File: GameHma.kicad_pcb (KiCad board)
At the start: 2 copper layers, 14 parts, among them J2 Motor_Terminal_01x04, J3 Motor_Terminal_01x04, J4 Motor_Terminal_01x04, J5 Motor_Terminal_01x04, U1 ESP32-DEVKIT-V1, U2 A4988_STEPPER_MOTOR_DRIVER_CA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, U3 A4988_STEPPER_MOTOR_DRIVER_CA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, U4 A4988_STEPPER_MOTOR_DRIVER_CA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, U5 A4988_STEPPER_MOTOR_DRIVER_CA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, U6 SRT_MP1584EN

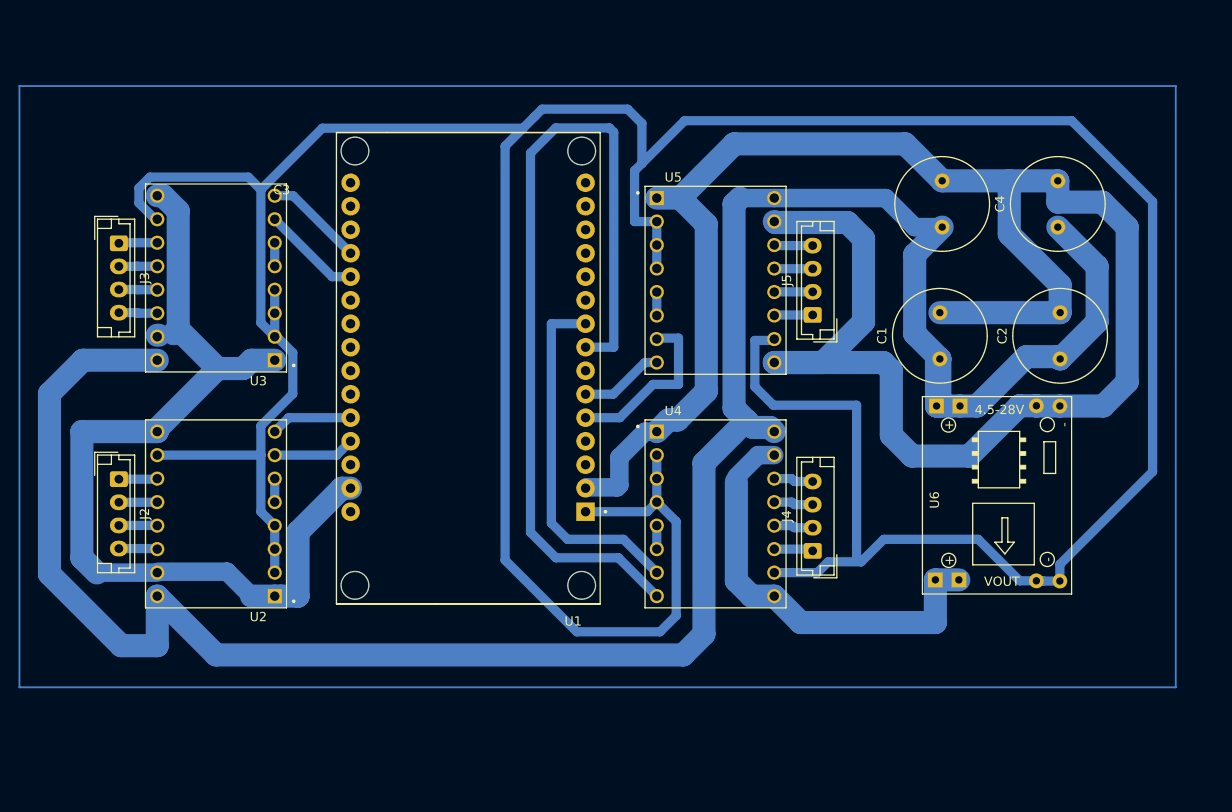
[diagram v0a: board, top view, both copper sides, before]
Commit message: Add log, Finish PCB rout line
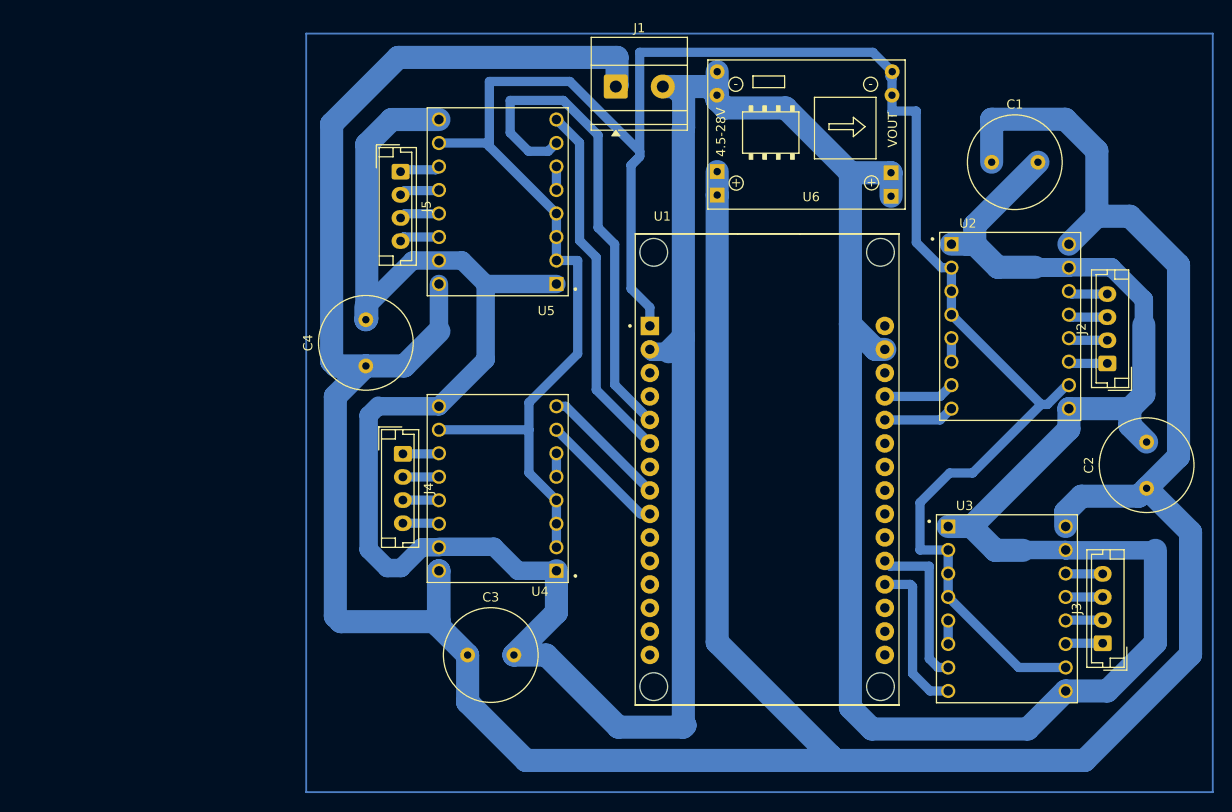
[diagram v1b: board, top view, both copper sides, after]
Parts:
- added J1: Screw_Terminal_01x02, TerminalBlock_Phoenix:TerminalBlock_Phoenix_MKDS-1,5-2-5.08_1x02_P5.08mm_Horizontal, F.Cu at (130.2, 64.8)
- moved J3 114.8 mm to (182.8, 125.0), turned to 90 degrees
- moved J2 107.6 mm to (183.3, 94.7), turned to 90 degrees
- moved U3 92.7 mm to (172.5, 121.3), turned to 0 degrees
- moved U2 88.2 mm to (172.8, 90.7), turned to 0 degrees
- moved C4 76.3 mm to (103.2, 95.0)
- moved C3 69.1 mm to (114.2, 126.3), turned to 0 degrees
- moved J5 47.2 mm to (107.0, 74.0), turned to -90 degrees
- moved J4 45.5 mm to (107.2, 104.5), turned to -90 degrees
- moved U6 45.1 mm to (151.3, 69.4), turned to 0 degrees
- moved U1 34.2 mm to (146.6, 106.2), turned to 0 degrees
- moved U5 25.0 mm to (117.5, 77.3), turned to 180 degrees
- moved U4 23.7 mm to (117.5, 108.3), turned to 180 degrees
- moved C1 22.0 mm to (170.8, 73.0), turned to 0 degrees
- moved C2 16.8 mm to (187.6, 108.2)
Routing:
- net +V_{DD}: track 416.3 -> 250.0 mm
- net +V_{batt}: track 252.3 -> 392.9 mm
- net GND: track 375.4 -> 468.3 mm
- net DIR_3: track 94.1 -> 13.9 mm
- net STEP_4: track 18.9 -> 53.9 mm
- net DIR_4: track 9.12 -> 39.2 mm
- net STEP_3: track 38.9 -> 13.9 mm
- net STEP_1: track 10.8 -> 17.5 mm
- net DIR_1: track 10.8 -> 17.1 mm
- net STEP_2: track 8.82 -> 7.71 mm
- net DIR_2: track 8.82 -> 7.71 mm
